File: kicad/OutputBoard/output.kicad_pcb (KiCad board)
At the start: 2 copper layers, 60.3 x 139.1 mm, 117 parts, among them J1 MAIN_BOARD_IO, J2 MAIN_BOARD_POWER, J3 MAIN_BOARD_FP, J4 Serial (3v3), Q1 AO3400A, Q10 AO3400A, Q11 IRF9Z24NPBF, Q12 AO3400A, Q2 IRF9Z24NPBF, Q3 AO3400A, Q4 AO3400A, Q5 IRF9Z24NPBF, Q6 AO3400A, Q7 AO3400A, Q8 IRF9Z24NPBF, Q9 AO3400A, U1 LM324, U2 MCP4728, U3 TPS5430DDA, U4 Pico, U5 XC6206P332MR

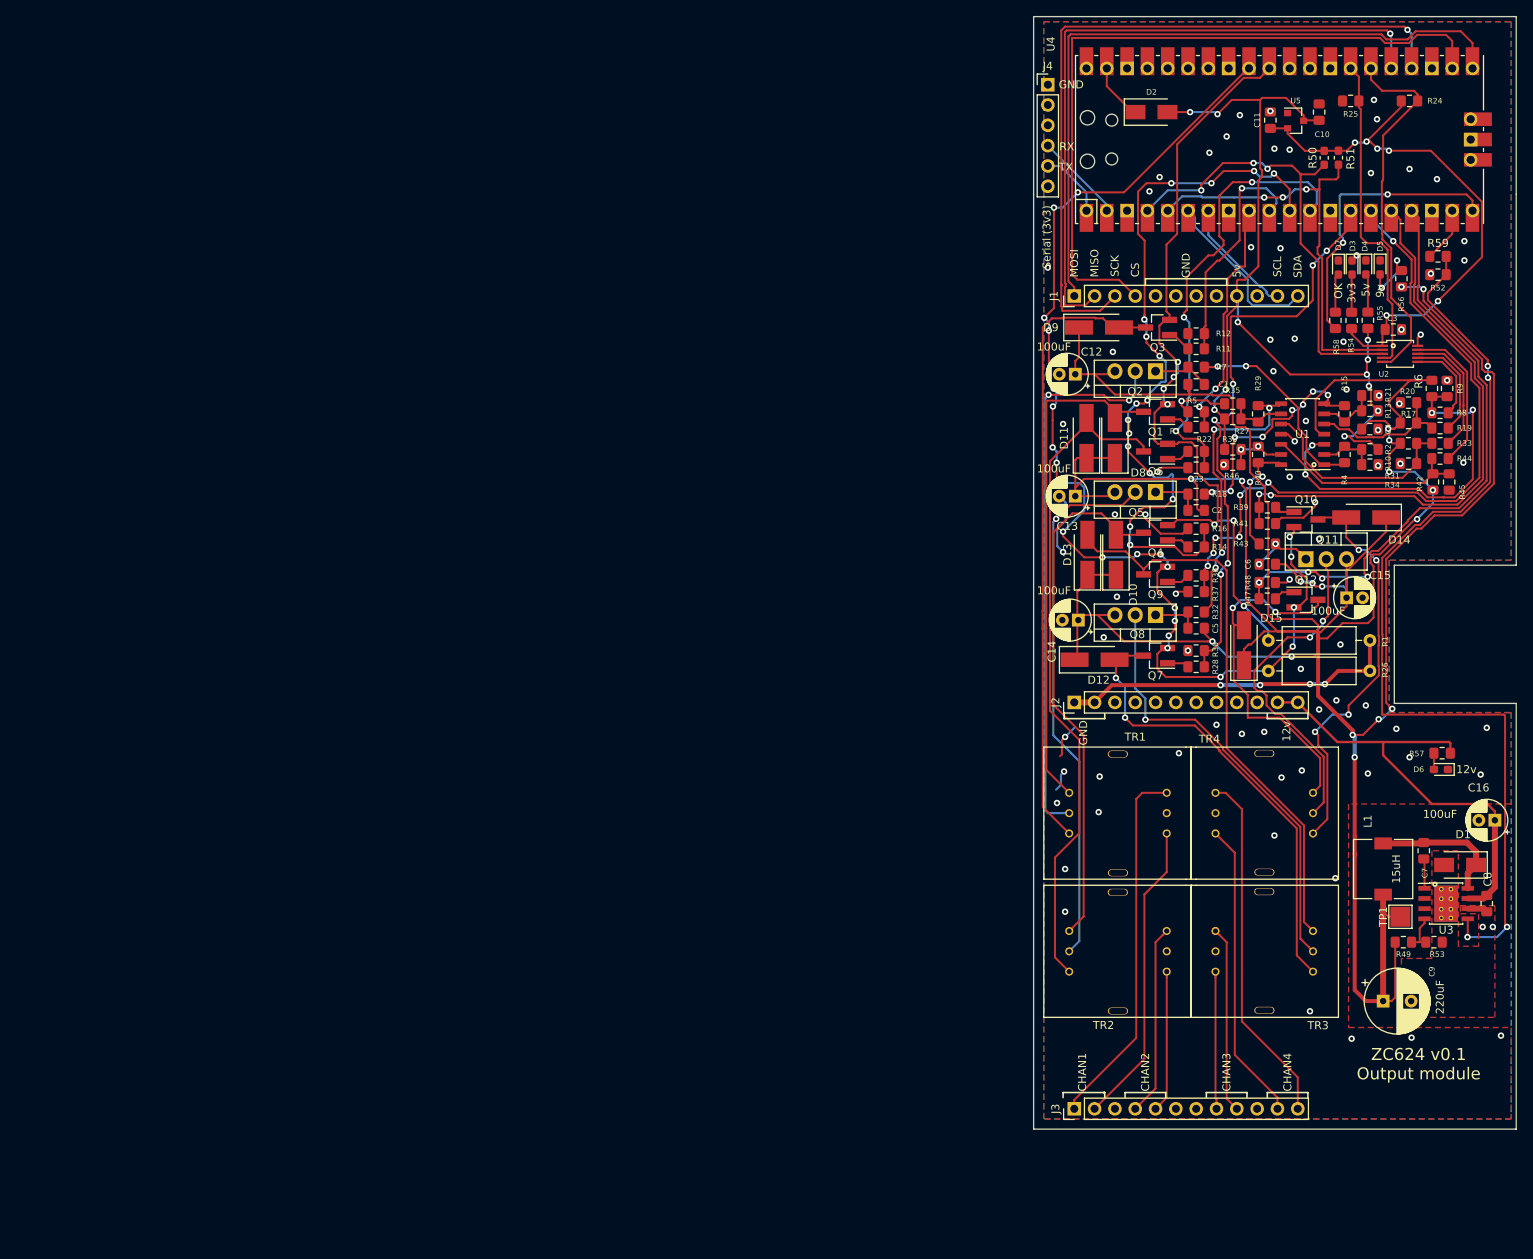
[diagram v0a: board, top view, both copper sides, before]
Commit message: Update kicad project
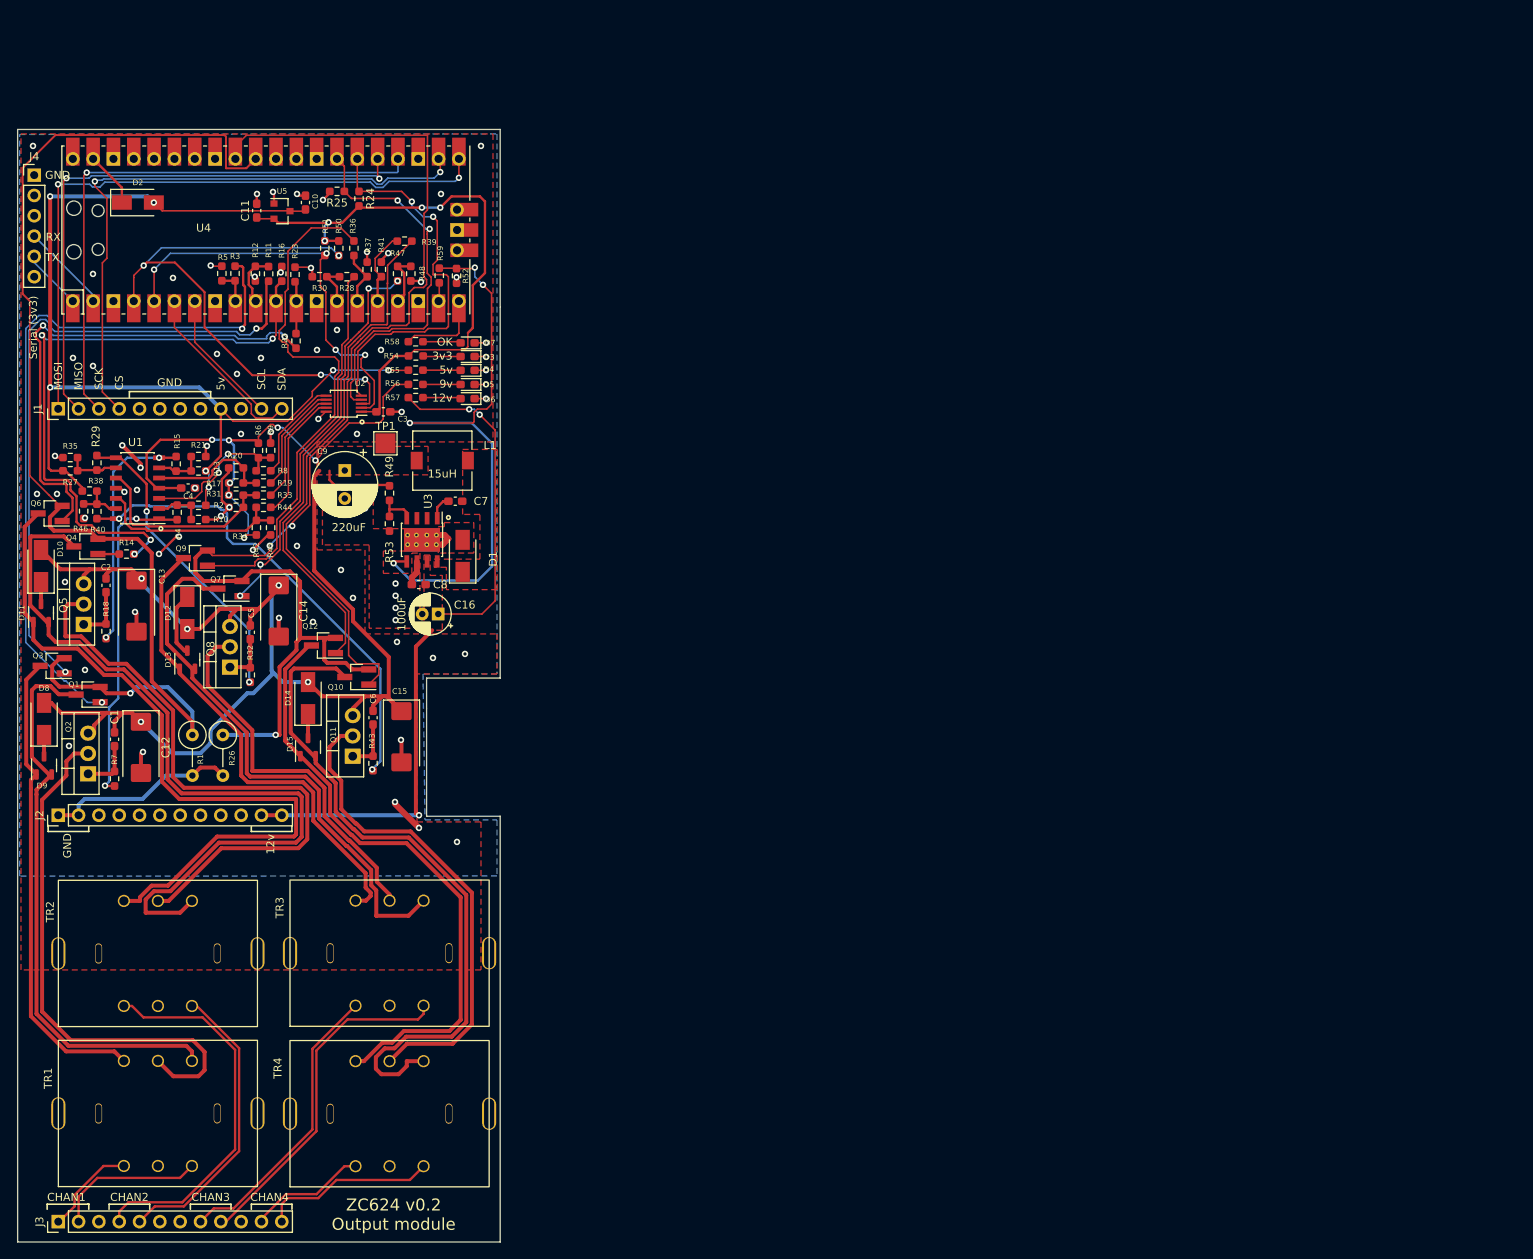
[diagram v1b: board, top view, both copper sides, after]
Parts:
- C1, C10, C11, C2, C3, C4, C5, C6, C7, C8: footprint Capacitor_SMD:C_0805_2012Metric_Pad1.15x1.40mm_HandSolder -> Capacitor_SMD:C_0603_1608Metric_Pad1.08x0.95mm_HandSolder
- C12, C13, C14, C15: value 100uF -> 220uF; footprint Capacitor_THT:CP_Radial_D5.0mm_P2.00mm -> Capacitor_Tantalum_SMD:CP_EIA-7343-43_Kemet-X_Pad2.25x2.55mm_HandSolder
- D10, D12, D14, D8: value SS210 -> SMAJ13A; footprint Diode_SMD:D_SMA_Handsoldering -> Diode_SMD:D_SMA
- D11, D13, D15, D9: value SS210 -> BAV23CL; footprint Diode_SMD:D_SMA_Handsoldering -> Package_TO_SOT_SMD:SOT-23-3
- R1, R26: footprint Resistor_THT:R_Axial_DIN0309_L9.0mm_D3.2mm_P12.70mm_Horizontal -> Resistor_THT:R_Axial_DIN0309_L9.0mm_D3.2mm_P5.08mm_Vertical
- R10, R11, R12, R13, R14, R15, R16, R17, R18, R19, R2, R20, R21, R22, R23, R24, R25, R27, R28, R29, R3, R30, R31, R32, R33, R34, R35, R36, R37, R38, R39, R4, R40, R41, R42, R43, R44, R45, R46, R47, R48, R49, R5, R52, R53, R59, R6, R7, R8, R9: footprint Resistor_SMD:R_0805_2012Metric_Pad1.15x1.40mm_HandSolder -> Resistor_SMD:R_0603_1608Metric_Pad0.98x0.95mm_HandSolder
- R50, R51: footprint Resistor_SMD:R_0603_1608Metric_Pad1.05x0.95mm_HandSolder -> Resistor_SMD:R_0603_1608Metric_Pad0.98x0.95mm_HandSolder
- R54, R58: value 680 -> 1.5k; footprint Resistor_SMD:R_0805_2012Metric_Pad1.15x1.40mm_HandSolder -> Resistor_SMD:R_0603_1608Metric_Pad0.98x0.95mm_HandSolder
- R55: value 1k -> 4k7; footprint Resistor_SMD:R_0805_2012Metric_Pad1.15x1.40mm_HandSolder -> Resistor_SMD:R_0603_1608Metric_Pad0.98x0.95mm_HandSolder
- R56: value 1.8k -> 10k; footprint Resistor_SMD:R_0805_2012Metric_Pad1.15x1.40mm_HandSolder -> Resistor_SMD:R_0603_1608Metric_Pad0.98x0.95mm_HandSolder
- R57: value 2.7k -> 10k; footprint Resistor_SMD:R_0805_2012Metric_Pad1.15x1.40mm_HandSolder -> Resistor_SMD:R_0603_1608Metric_Pad0.98x0.95mm_HandSolder
- TR1, TR2, TR3, TR4: footprint out:42TL004-RC -> out:42TL+U
- moved C4 147.9 mm to (89.9, 72.3)
- moved R45 147.4 mm to (100.2, 77.2)
- moved R9 147.3 mm to (100.2, 67.6)
- moved R8 147.2 mm to (99.3, 70.1)
- moved R19 147.2 mm to (99.3, 71.6)
- moved R33 147.2 mm to (99.3, 73.2)
- moved R44 147.2 mm to (99.3, 74.7)
- moved R42 147.2 mm to (98.4, 77.2)
- moved R6 146.9 mm to (98.7, 67.6)
- moved R20 146.8 mm to (95.9, 69.8)
- moved R17 146.7 mm to (95.9, 71.6)
- moved R31 146.7 mm to (95.9, 73.2)
- moved R34 146.7 mm to (95.9, 74.7)
- moved R21 146.6 mm to (91.2, 68.3)
- moved R13 146.6 mm to (91.2, 70.1)
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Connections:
- D10 pad 1: +9v -> Net-(D10-Pad1)
- D10 pad 2: Net-(D10-Pad2) -> +9v
- D11 pad 1: +9v -> Net-(D11-Pad1)
- D12 pad 1: +9v -> Net-(D12-Pad1)
- D12 pad 2: Net-(D12-Pad2) -> +9v
- D13 pad 1: +9v -> Net-(D13-Pad1)
- D14 pad 1: +9v -> Net-(D14-Pad1)
- D14 pad 2: Net-(D14-Pad2) -> +9v
- D15 pad 1: +9v -> Net-(D15-Pad1)
- D8 pad 1: +9v -> Net-(D8-Pad1)
- D8 pad 2: Net-(D8-Pad2) -> +9v
- D9 pad 1: +9v -> Net-(D9-Pad1)
- J1 pad 10: (no net) -> unconnected-(J1-Pad10)
- J2 pad 10: (no net) -> unconnected-(J2-Pad10)
- J2 pad 3: (no net) -> unconnected-(J2-Pad3)
- J2 pad 4: (no net) -> unconnected-(J2-Pad4)
- J2 pad 5: (no net) -> unconnected-(J2-Pad5)
- J2 pad 6: (no net) -> unconnected-(J2-Pad6)
- J2 pad 7: (no net) -> unconnected-(J2-Pad7)
- J2 pad 8: (no net) -> unconnected-(J2-Pad8)
- J2 pad 9: (no net) -> unconnected-(J2-Pad9)
- J3 pad 1: Net-(J3-Pad1) -> C1-OUT-A
- J3 pad 10: (no net) -> unconnected-(J3-Pad10)
- J3 pad 11: Net-(J3-Pad11) -> C4-OUT-A
- J3 pad 12: Net-(J3-Pad12) -> C4-OUT-B
- J3 pad 2: Net-(J3-Pad2) -> C1-OUT-B
- J3 pad 3: (no net) -> unconnected-(J3-Pad3)
- J3 pad 4: Net-(J3-Pad4) -> C2-OUT-A
- J3 pad 5: Net-(J3-Pad5) -> C2-OUT-B
- J3 pad 6: (no net) -> unconnected-(J3-Pad6)
- J3 pad 7: (no net) -> unconnected-(J3-Pad7)
- J3 pad 8: Net-(J3-Pad8) -> C3-OUT-A
- J3 pad 9: Net-(J3-Pad9) -> C3-OUT-B
- J4 pad 2: (no net) -> unconnected-(J4-Pad2)
- J4 pad 3: (no net) -> unconnected-(J4-Pad3)
- J4 pad 6: (no net) -> unconnected-(J4-Pad6)
- Q1 pad 3: Net-(D8-Pad2) -> Net-(D9-Pad2)
- Q10 pad 3: Net-(D14-Pad2) -> Net-(D15-Pad2)
- Q12 pad 3: Net-(D15-Pad2) -> Net-(D15-Pad1)
- Q3 pad 3: Net-(D9-Pad2) -> Net-(D9-Pad1)
- Q4 pad 3: Net-(D10-Pad2) -> Net-(D11-Pad2)
- Q6 pad 3: Net-(D11-Pad2) -> Net-(D11-Pad1)
- Q7 pad 3: Net-(D12-Pad2) -> Net-(D13-Pad2)
- Q9 pad 3: Net-(D13-Pad2) -> Net-(D13-Pad1)
- R54 pad 1: +3v3 -> Net-(D3-Pad2)
- R54 pad 2: Net-(D3-Pad2) -> +3v3
- R56 pad 1: +9v -> Net-(D5-Pad2)
- R56 pad 2: Net-(D5-Pad2) -> +9v
- R57 pad 1: +12v -> Net-(D6-Pad2)
- R57 pad 2: Net-(D6-Pad2) -> +12v
- R58 pad 1: OK_LED -> Net-(D7-Pad2)
- R58 pad 2: Net-(D7-Pad2) -> OK_LED
- TR1 pad 1: Net-(D8-Pad2) -> Net-(D9-Pad2)
- TR1 pad 3: Net-(D9-Pad2) -> Net-(D9-Pad1)
- TR1 pad 4: Net-(J3-Pad2) -> C1-OUT-A
- TR1 pad 5: (no net) -> unconnected-(TR1-Pad5)
- TR1 pad 6: Net-(J3-Pad1) -> C1-OUT-B
- TR2 pad 1: Net-(D10-Pad2) -> Net-(D11-Pad2)
- TR2 pad 3: Net-(D11-Pad2) -> Net-(D11-Pad1)
- TR2 pad 4: Net-(J3-Pad5) -> C2-OUT-A
- TR2 pad 5: (no net) -> unconnected-(TR2-Pad5)
- TR2 pad 6: Net-(J3-Pad4) -> C2-OUT-B
- TR3 pad 1: Net-(D12-Pad2) -> Net-(D13-Pad2)
- TR3 pad 3: Net-(D13-Pad2) -> Net-(D13-Pad1)
- TR3 pad 4: Net-(J3-Pad9) -> C3-OUT-A
- TR3 pad 5: (no net) -> unconnected-(TR3-Pad5)
- TR3 pad 6: Net-(J3-Pad8) -> C3-OUT-B
- TR4 pad 1: Net-(D14-Pad2) -> Net-(D15-Pad2)
- TR4 pad 3: Net-(D15-Pad2) -> Net-(D15-Pad1)
- TR4 pad 4: Net-(J3-Pad12) -> C4-OUT-A
- TR4 pad 5: (no net) -> unconnected-(TR4-Pad5)
- TR4 pad 6: Net-(J3-Pad11) -> C4-OUT-B
- U3 pad 2: (no net) -> unconnected-(U3-Pad2)
- U3 pad 3: (no net) -> unconnected-(U3-Pad3)
- U4 pad 29: Net-(U4-Pad29) -> unconnected-(U4-Pad29)
- U4 pad 30: Net-(U4-Pad30) -> unconnected-(U4-Pad30)
- U4 pad 33: Net-(U4-Pad33) -> unconnected-(U4-Pad33)
- U4 pad 34: Net-(U4-Pad34) -> unconnected-(U4-Pad34)
- U4 pad 35: Net-(U4-Pad35) -> unconnected-(U4-Pad35)
- U4 pad 36: Net-(U4-Pad36) -> unconnected-(U4-Pad36)
- U4 pad 37: Net-(U4-Pad37) -> unconnected-(U4-Pad37)
- U4 pad 40: Net-(U4-Pad40) -> unconnected-(U4-Pad40)
- U4 pad 41: Net-(U4-Pad41) -> unconnected-(U4-Pad41)
- U4 pad 42: Net-(U4-Pad42) -> unconnected-(U4-Pad42)
- U4 pad 43: Net-(U4-Pad43) -> unconnected-(U4-Pad43)
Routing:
- net +9v: track 461.4 -> 235.0 mm, vias 18 -> 12
- net Net-(D11-Pad1): track 0.00 -> 92.6 mm
- net Net-(Q1-Pad1): track 3.39 -> 89.5 mm, vias 0 -> 2
- net C3-GB: track 87.6 -> 6.91 mm, vias 7 -> 0
- net Net-(Q3-Pad1): track 3.00 -> 82.0 mm, vias 0 -> 2
- net Net-(D15-Pad1): track 0.00 -> 76.2 mm
- net C4-GB: track 76.2 -> 6.66 mm, vias 4 -> 0
- net C3-GA: track 73.2 -> 5.16 mm, vias 6 -> 0
- net Net-(Q10-Pad1): track 2.53 -> 70.1 mm
- net Net-(D10-Pad2): track 66.3 -> 0.00 mm
- net Net-(Q9-Pad1): track 2.89 -> 67.1 mm
- net Net-(D8-Pad2): track 64.1 -> 0.00 mm
- net C4-GA: track 72.0 -> 9.41 mm, vias 2 -> 0
- net Net-(D13-Pad1): track 0.00 -> 60.3 mm
- net Net-(Q6-Pad1): track 2.94 -> 62.5 mm, vias 0 -> 2
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- added copper zone on F.Cu, net +12v
- added copper zone on F.Cu, net +9v
- added copper zone on F.Cu, net Net-(C7-Pad1)
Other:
- outline, holes or cut-outs redrawn
- net class Default removed
- board text added: "ZC624 v0.2 Output module"
- board text removed: "ZC624 v0.1 Output module"
